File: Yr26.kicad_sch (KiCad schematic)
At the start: 0 parts

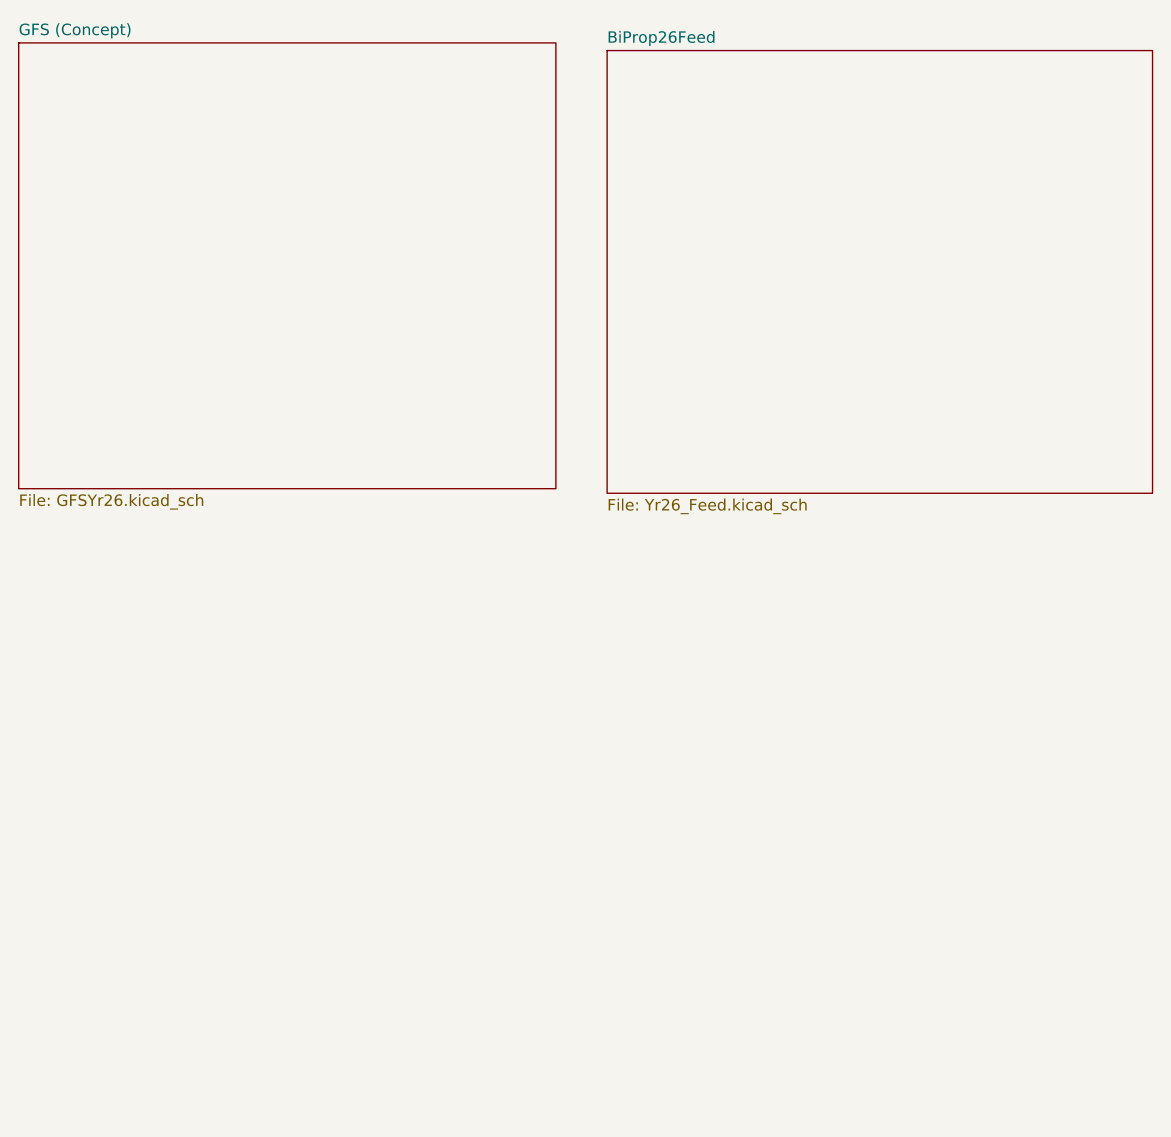
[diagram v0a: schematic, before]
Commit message: feedfeed
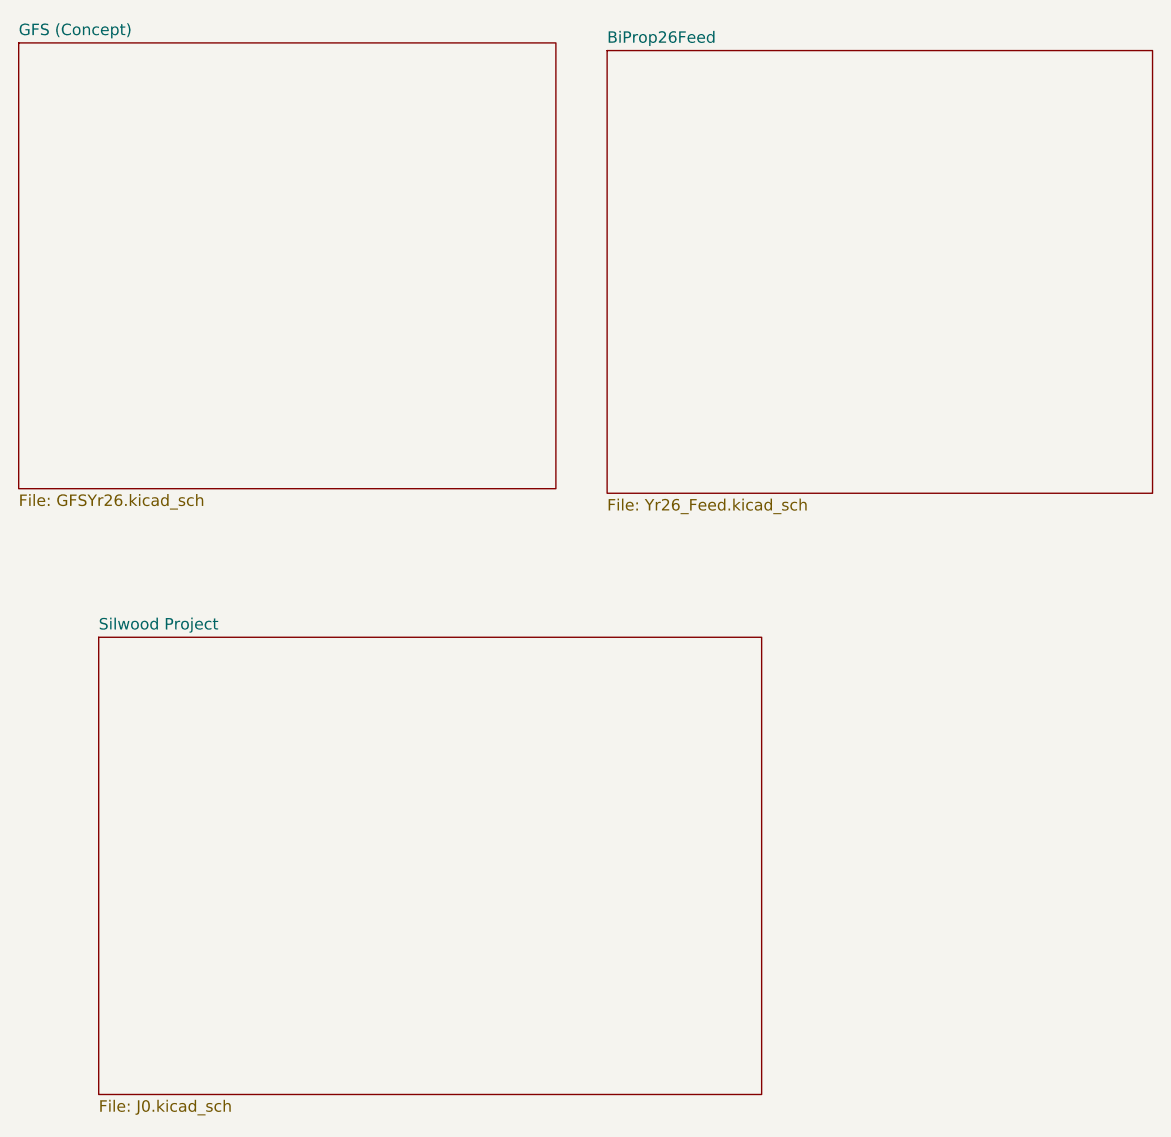
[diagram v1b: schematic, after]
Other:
- added sheet Silwood Project (J0.kicad_sch)
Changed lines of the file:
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@@
+		)
+	)
+	(sheet
+		(at 25.4 82.55)
+		(size 73.66 50.8)
+		(exclude_from_sim no)
+		(in_bom yes)
+		(on_board yes)
+		(dnp no)
+		(fields_autoplaced yes)
+		(stroke
+			(width 0.1524)
+			(type solid)
+		)
+		(fill
+			(color 0 0 0 0.0000)
+		)
+		(property "Sheetname" "Silwood Project"
+			(at 25.4 81.8384 0)
+			(effects
+				(font
+					(size 1.27 1.27)
+				)
+				(justify left bottom)
+			)
+		)
+		(property "Sheetfile" "J0.kicad_sch"
+			(at 25.4 133.9346 0)
+			(effects
+				(font
+					(size 1.27 1.27)
+				)
+				(justify left top)
+			)
+		)
+		(instances
+			(project "P_IDs"
+				(path "/045f1f05-3134-4b6d-91b6-463031104f1e/a0b6300e-76e9-4a18-afd6-e2d656b0d8f9"
+					(page "21")
+				)
+			)
 		)
 	)

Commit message: andrei it support
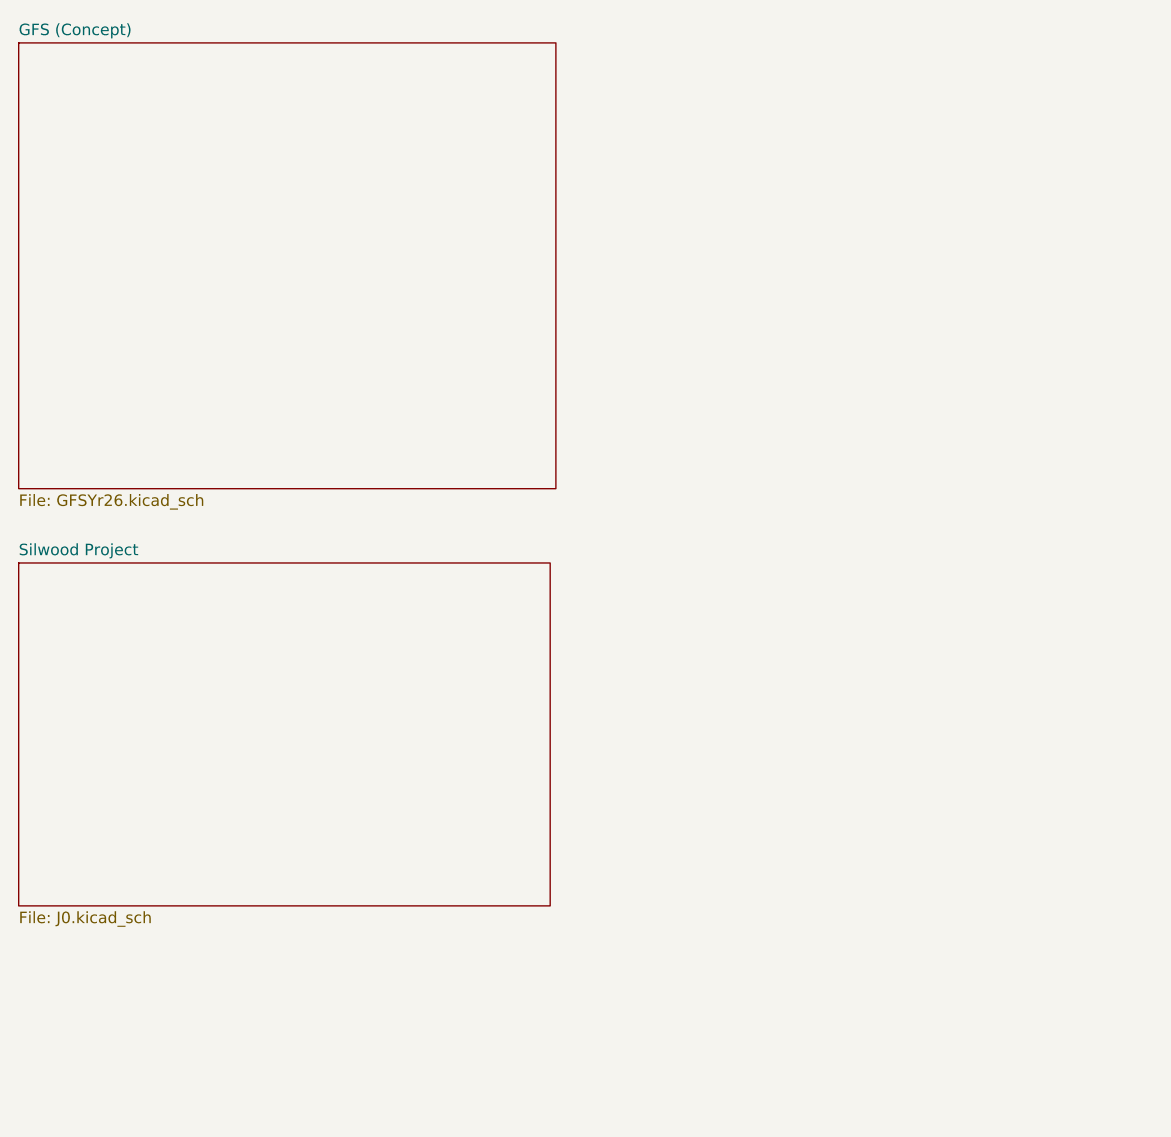
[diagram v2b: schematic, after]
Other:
- removed sheet BiProp26Feed
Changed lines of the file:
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@@
 	)
 	(sheet
-		(at 81.892 17.3601)
-		(size 60.602 49.1879)
+		(at 16.51 74.295)
+		(size 59.055 38.1)
 		(exclude_from_sim no)
 		(in_bom yes)
@@
 			(color 0 0 0 0.0000)
 		)
-		(property "Sheetname" "BiProp26Feed"
-			(at 81.892 16.6485 0)
+		(property "Sheetname" "Silwood Project"
+			(at 16.51 73.5834 0)
 			(effects
 				(font
@@
 			)
 		)
-		(property "Sheetfile" "Yr26_Feed.kicad_sch"
-			(at 81.892 67.1326 0)
+		(property "Sheetfile" "J0.kicad_sch"
+			(at 16.51 112.9796 0)
 			(effects
 				(font
@@
 				)
 			)
-		)
-	)
-	(sheet
-		(at 25.4 82.55)
-		(size 73.66 50.8)
-		(exclude_from_sim no)
-		(in_bom yes)
-		(on_board yes)
-		(dnp no)
-		(fields_autoplaced yes)
-		(stroke
-			(width 0.1524)
-			(type solid)
-		)
-		(fill
-			(color 0 0 0 0.0000)
-		)
-		(property "Sheetname" "Silwood Project"
-			(at 25.4 81.8384 0)
-			(effects
-				(font
-					(size 1.27 1.27)
-				)
-				(justify left bottom)
-			)
-		)
-		(property "Sheetfile" "J0.kicad_sch"
-			(at 25.4 133.9346 0)
-			(effects
-				(font
-					(size 1.27 1.27)
-				)
-				(justify left top)
-			)
-		)
-		(instances
-			(project "P_IDs"
-				(path "/045f1f05-3134-4b6d-91b6-463031104f1e/a0b6300e-76e9-4a18-afd6-e2d656b0d8f9"
-					(page "21")
-				)
-			)

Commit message: Feediddy
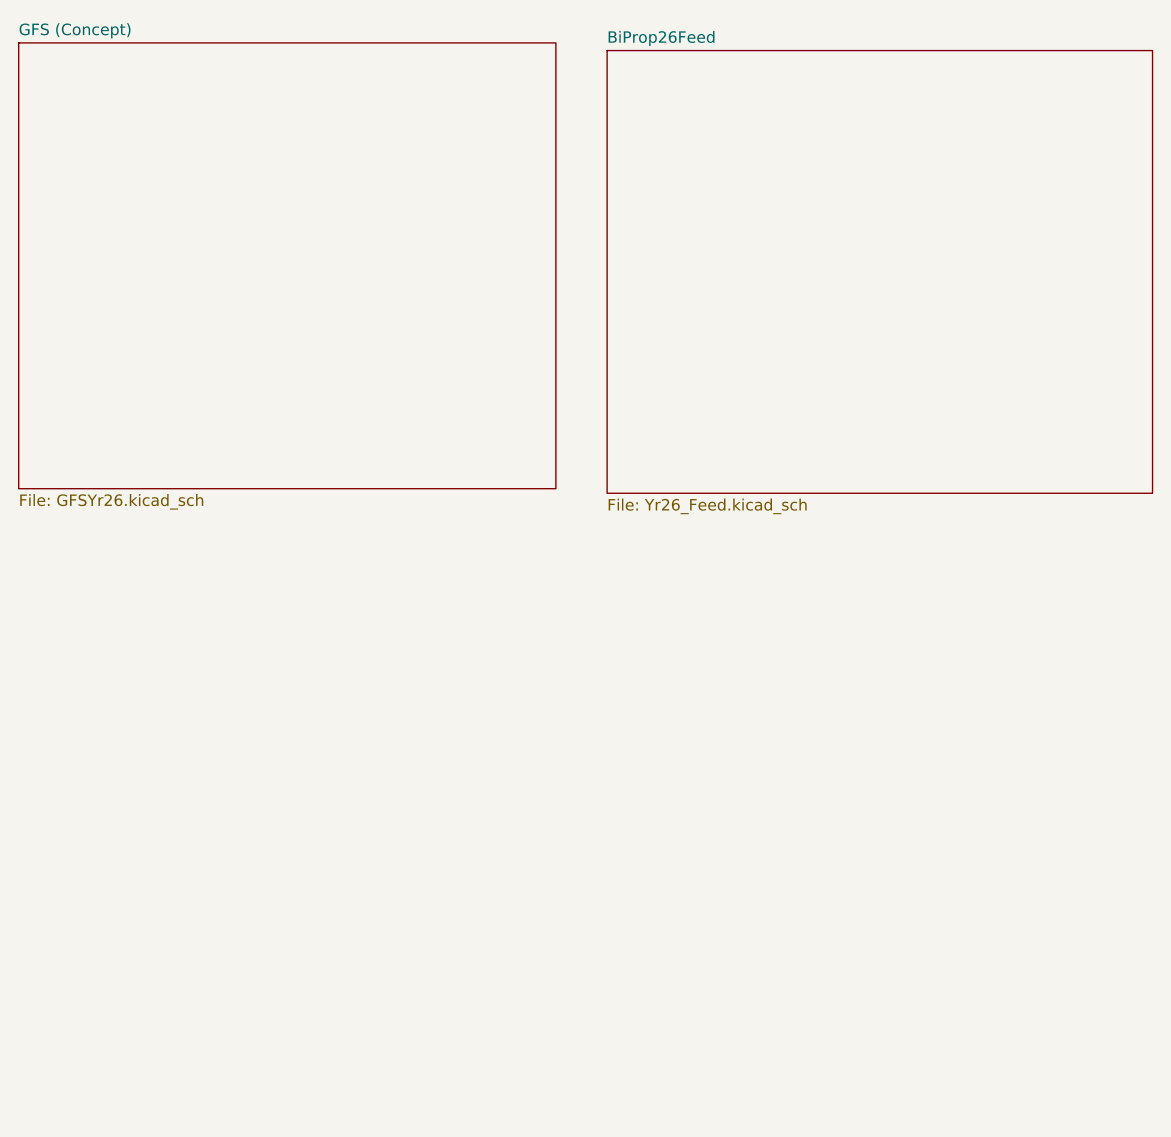
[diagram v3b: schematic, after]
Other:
- removed sheet Silwood Project
- added sheet BiProp26Feed (Yr26_Feed.kicad_sch)
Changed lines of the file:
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@@
 	)
 	(sheet
-		(at 16.51 74.295)
-		(size 59.055 38.1)
+		(at 81.892 17.3601)
+		(size 60.602 49.1879)
 		(exclude_from_sim no)
 		(in_bom yes)
@@
 			(color 0 0 0 0.0000)
 		)
-		(property "Sheetname" "Silwood Project"
-			(at 16.51 73.5834 0)
+		(property "Sheetname" "BiProp26Feed"
+			(at 81.892 16.6485 0)
 			(effects
 				(font
@@
 			)
 		)
-		(property "Sheetfile" "J0.kicad_sch"
-			(at 16.51 112.9796 0)
+		(property "Sheetfile" "Yr26_Feed.kicad_sch"
+			(at 81.892 67.1326 0)
 			(effects
 				(font
